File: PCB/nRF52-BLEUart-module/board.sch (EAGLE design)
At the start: 2 parts, among them J1 USB-A_PTH_MALE, U1 NRF52832

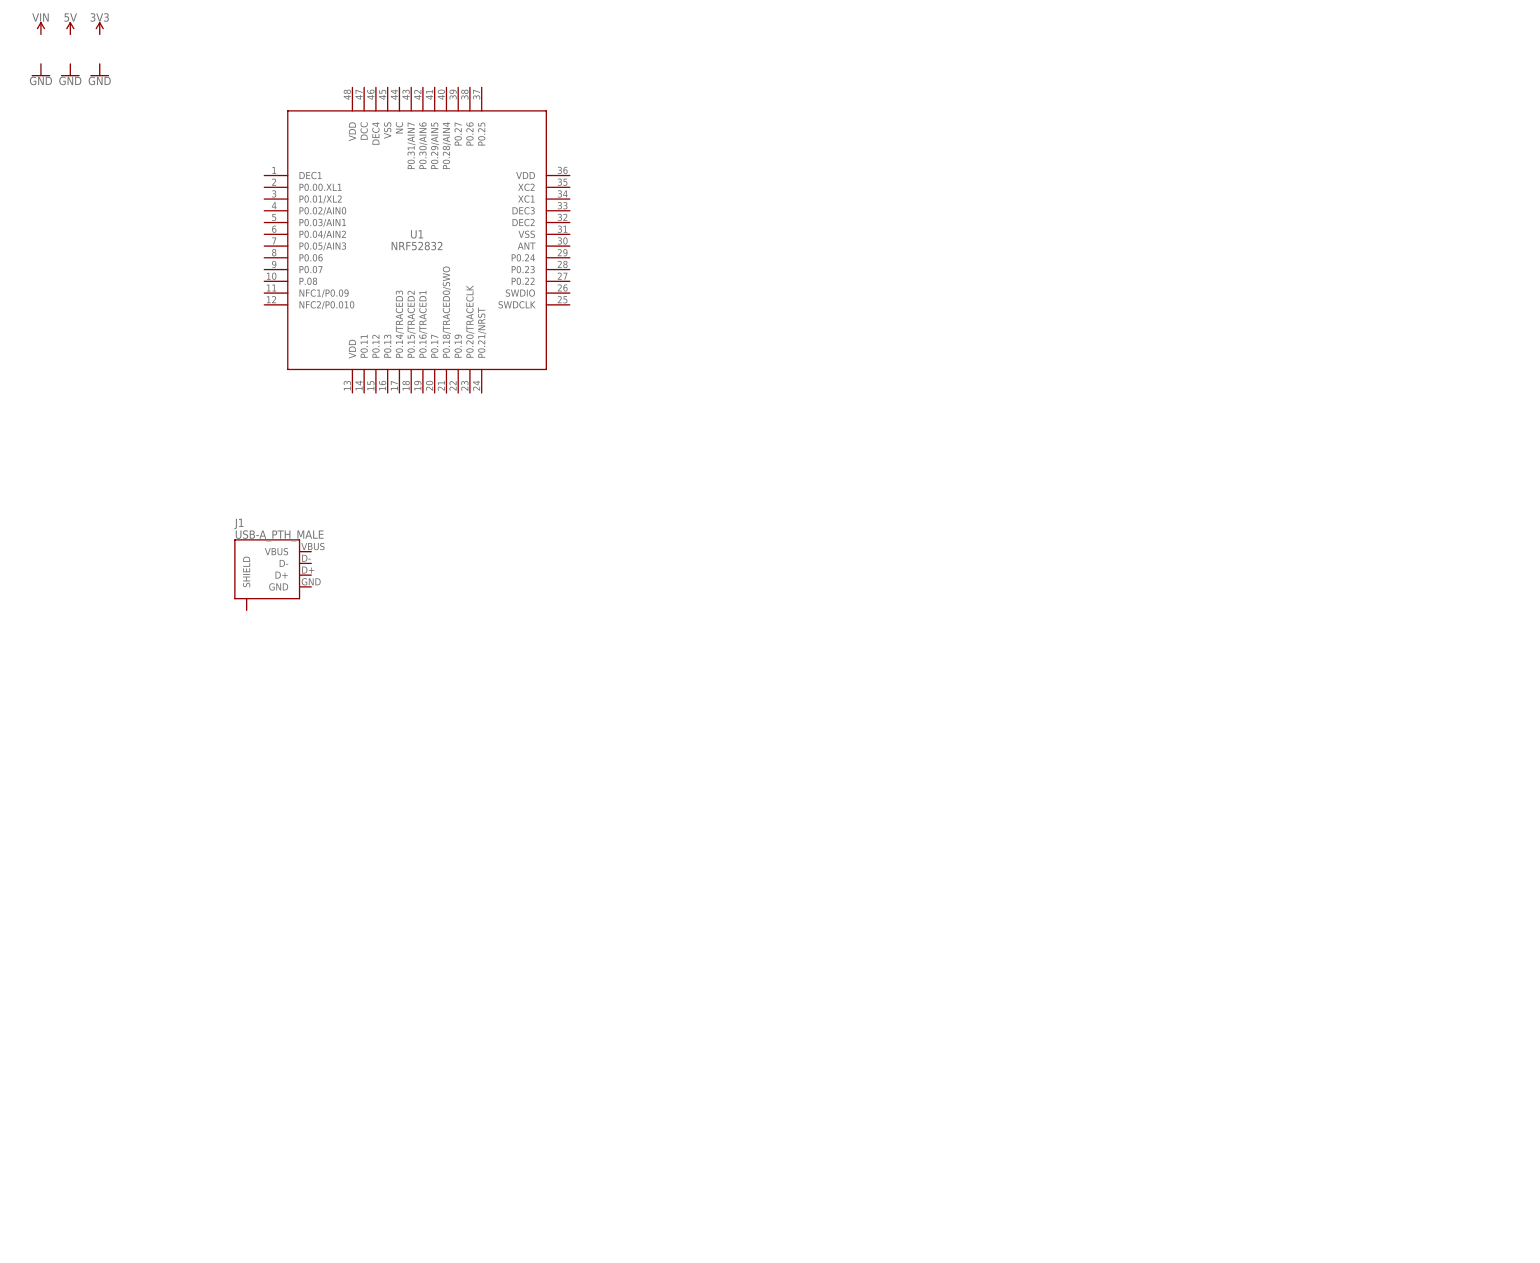
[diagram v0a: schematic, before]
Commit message: PCB update
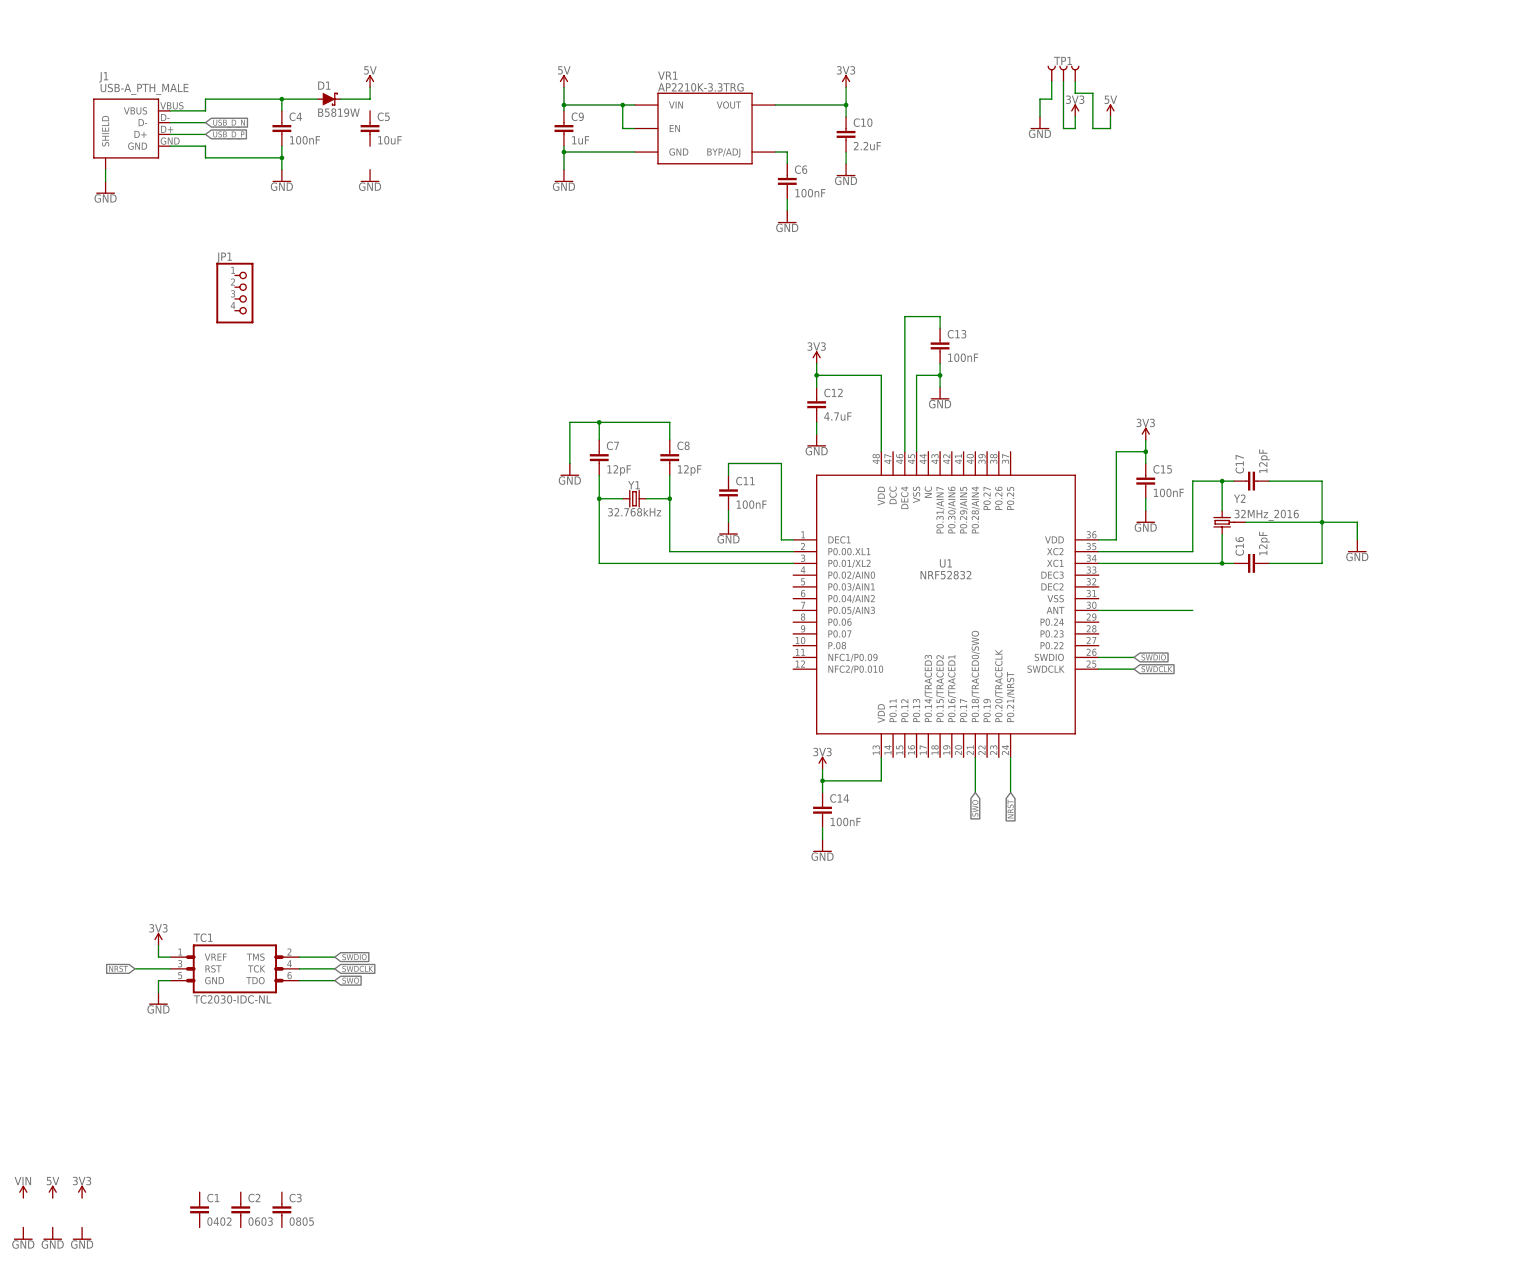
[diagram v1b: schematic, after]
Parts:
- added C1: 0402, angrypig7-RCL:C-NON-POLC0402
- added C10: 2.2uF, angrypig7-RCL:C-NON-POLC0603
- added C11, C13, C14, C15, C4, C6: 100nF, angrypig7-RCL:C-NON-POLC0402
- added C12: 4.7uF, angrypig7-RCL:C-NON-POLC0402
- added C16, C17, C7, C8: 12pF, angrypig7-RCL:C-NON-POLC0402
- added C2: 0603, angrypig7-RCL:C-NON-POLC0603
- added C3: 0805, angrypig7-RCL:C-NON-POLC0805
- added C5: 10uF, angrypig7-RCL:C-NON-POLC0603
- added C9: 1uF, angrypig7-RCL:C-NON-POLC0402
- added D1: B5819W, angrypig7-Diodes:DIODE-SCHOTTKY_SOD-123
- added JP1: (no value), angrypig7-Connectors-PinHeads:PINHD-1X4
- added TC1: TC2030-IDC-NL, angrypig7-Connectors-Programming:TC2030-IDC-NL
- added TP1: TEST-POINT-3, angrypig7-Tests:TEST-POINT-3
- added VR1: AP2210K-3.3TRG, angrypig7-IC-Power:AP2210K
- added Y1: 32.768kHz, angrypig7-Clocks:CRYSTAL-32.768KHZ_3215
- added Y2: 32MHz_2016, angrypig7-Clocks:CRYSTAL-2.0X1.6MM
- J1: LCSC (none) -> C98125
- U1: LCSC (none) -> C77540
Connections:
- new net 3V3: C10.1, C12.1, C14.1, C15.1, TC1.VREF, TP1.2, U1.VDD@0, U1.VDD@1, U1.VDD@2, VR1.VOUT
- new net 5V: C9.1, D1.C, TP1.3, VR1.EN, VR1.VIN
- new net GND: C10.2, C11.2, C12.2, C13.2, C14.2, C15.2, C16.2, C17.2, C4.2, C6.2, C7.1, C8.1, C9.2, J1.GND, J1.SHIELD, TC1.GND, TP1.1, U1.VSS@1, VR1.GND, Y2.GND
- new net N$1: C8.2, U1.P0.00.XL1, Y1.2
- new net N$2: C4.1, D1.A, J1.VBUS
- new net N$3: C6.1, VR1.BYP/ADJ
- new net N$4: C7.2, U1.P0.01/XL2, Y1.1
- new net N$5: C11.1, U1.DEC1
- new net N$6: U1.ANT
- new net N$7: C13.1, U1.DEC4
- new net N$8: C17.1, U1.XC2, Y2.2
- new net N$9: C16.1, U1.XC1, Y2.1
- new net NRST: TC1.RST, U1.P0.21/NRST
- new net SWDCLK: TC1.TCK, U1.SWDCLK
- new net SWDIO: TC1.TMS, U1.SWDIO
- new net SWO: TC1.TDO, U1.P0.18/TRACED0/SWO
- new net USB_D_N: J1.D-
- new net USB_D_P: J1.D+
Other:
- moved on the sheet: J1, U1

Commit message: PCB update
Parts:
- added D2: TVS, angrypig7-Diodes:TVS-ARRAY_SOT-23-6
- added D3, D4, D5, D6: 0603, angrypig7-Diodes:LED_0603
- added L1: (no value), angrypig7-RCL:L0402
- added R1, R2, R3, R4, R5: 10k, angrypig7-RCL:RR0402
- added S1: SPST-3x4mm, angrypig7-Switches:SWITCH-SPST-SMD-3.0X4.0MM
- added U2: NRF52832, angrypig7-IC-MCU:NRF52832
- C1: value 0402 -> 1uF; LCSC (none) -> C52923
- C10: value 2.2uF -> 100nF; device angrypig7-RCL:C-NON-POLC0603 -> angrypig7-RCL:C-NON-POLC0402; LCSC C23630 -> C1525
- C11, C6: value 100nF -> 12pF; LCSC C1525 -> C1547
- C12: value 4.7uF -> 100nF; LCSC C23733 -> C1525
- C13: value 100nF -> 100pF; LCSC C1525 -> C1546
- C14: value 100nF -> 1uF; LCSC C1525 -> C52923
- C15: value 100nF -> 0.8pF
- C16: value 12pF -> 0.8pF; LCSC C1547 -> C1525
- C17: value 12pF -> 100nF; LCSC C1547 -> C1525
- C2: value 0603 -> 2.2uF; LCSC (none) -> C23630
- C3: value 0805 -> 100nF; device angrypig7-RCL:C-NON-POLC0805 -> angrypig7-RCL:C-NON-POLC0402; LCSC (none) -> C1525
- C5: value 10uF -> 4.7uF; device angrypig7-RCL:C-NON-POLC0603 -> angrypig7-RCL:C-NON-POLC0402; LCSC C19702 -> C23733
- C9: value 1uF -> 100nF; LCSC C52923 -> C1525
- JP1: value (none) -> V G Rx Tx; device angrypig7-Connectors-PinHeads:PINHD-1X4 -> angrypig7-Connectors-PinHeads:PINHD-1X4/90
- U1: value NRF52832 -> CH340E; device angrypig7-IC-MCU:NRF52832 -> angrypig7-IC:CH340E; LCSC C77540 -> C99652
- Y1: value 32.768kHz -> 32MHz_2016; device angrypig7-Clocks:CRYSTAL-32.768KHZ_3215 -> angrypig7-Clocks:CRYSTAL-2.0X1.6MM; LCSC C32346 -> C255896
- Y2: value 32MHz_2016 -> 32.768kHz; device angrypig7-Clocks:CRYSTAL-2.0X1.6MM -> angrypig7-Clocks:CRYSTAL-32.768KHZ_3215; LCSC (none) -> C32346
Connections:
- removed net USB_D_N: J1.D-
- removed net USB_D_P: J1.D+
- new net N$10: C13.1, U2.DEC3
- new net N$11: U2.DEC2
- new net N$12: D4.A, R3.1
- new net N$13: D5.A, R4.1
- new net N$14: D6.A, R5.1
- new net RF-1: C15.1, L1.1, U2.ANT
- new net RF-2: C16.1, L1.2
- new net UART_RX: JP1.4, U1.RX
- new net UART_TX: JP1.3, U1.TX
- new net USB_N: D2.IO3, D2.IO4, J1.D-, U1.UD-
- new net USB_P: D2.IO1, D2.IO2, J1.D+, U1.UD+
- net 3V3: now also C17.1, C2.1, C5.1, C9.1, JP1.1, R1.2, R2.2, R3.2, R4.2, R5.2, U1.V3, U1.VCC, U2.VDD@0, U2.VDD@1, U2.VDD@2; no longer C10.1, C14.1, C15.1, U1.VDD@0, U1.VDD@1, U1.VDD@2
- net 5V: now also C1.1; no longer C9.1
- net GND: now also C1.2, C2.2, C3.2, C5.2, D2.VSS, D3.C, JP1.2, S1.1, U1.GND, U2.PAD, U2.VSS@0, U2.VSS@1, Y1.GND; no longer U1.VSS@1, Y2.GND
- net N$1: now also U2.P0.00.XL1, Y2.2; no longer U1.P0.00.XL1, Y1.2
- net N$2: now also D2.VCC; no longer C4.1
- net N$3: now also C3.1; no longer C6.1
- net N$4: now also U2.P0.01/XL2, Y2.1; no longer U1.P0.01/XL2, Y1.1
- net N$5: now also C10.1, U2.DEC1; no longer C11.1, U1.DEC1
- net N$6: now also D3.A, R1.1; no longer U1.ANT
- net N$7: now also C4.1, U2.DEC4; no longer C13.1, U1.DEC4
- net N$8: now also C6.1, U2.XC2, Y1.2; no longer C17.1, U1.XC2, Y2.2
- net N$9: now also C11.1, U2.XC1, Y1.1; no longer C16.1, U1.XC1, Y2.1
- net NRST: now also C14.1, R2.1, S1.2, U2.P0.21/NRST; no longer U1.P0.21/NRST
- net SWDCLK: now also U2.SWDCLK; no longer U1.SWDCLK
- net SWDIO: now also U2.SWDIO; no longer U1.SWDIO
- net SWO: now also U2.P0.18/TRACED0/SWO; no longer U1.P0.18/TRACED0/SWO
